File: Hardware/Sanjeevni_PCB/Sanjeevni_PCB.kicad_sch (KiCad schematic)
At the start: 45 parts, among them J1 Conn_01x02, J2 Conn_01x04, J3 Conn_01x04, SW1 SW_Push, SW2 SW_Push, U1 AMS1117-3.3, U2 MT3608, U3 ADXL343, U4 ESP32-WROOM-32, U5 DHT11, U6 MQ-6

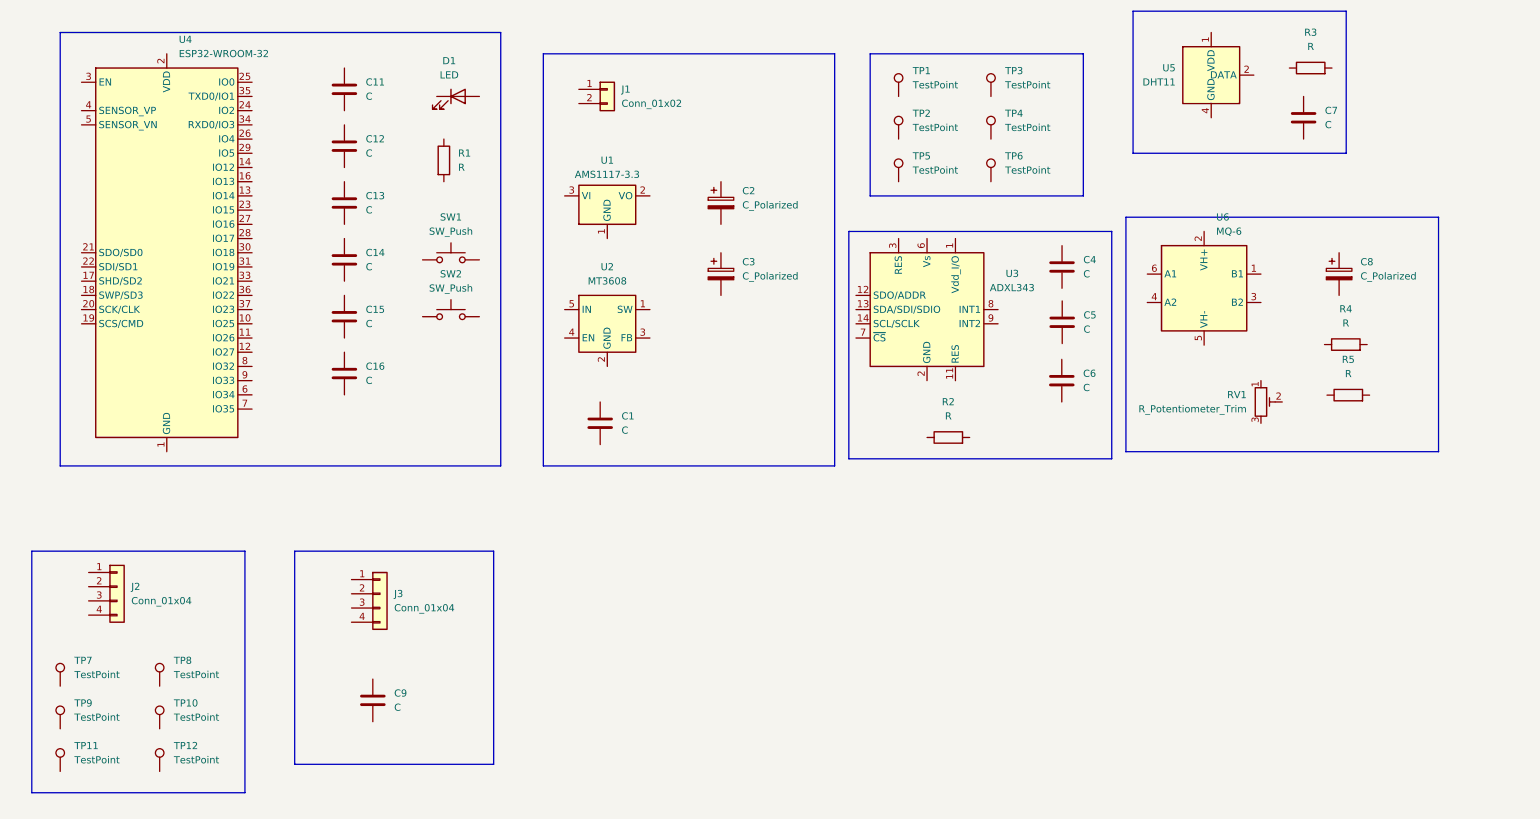
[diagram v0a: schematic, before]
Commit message: final PCB design KiCad
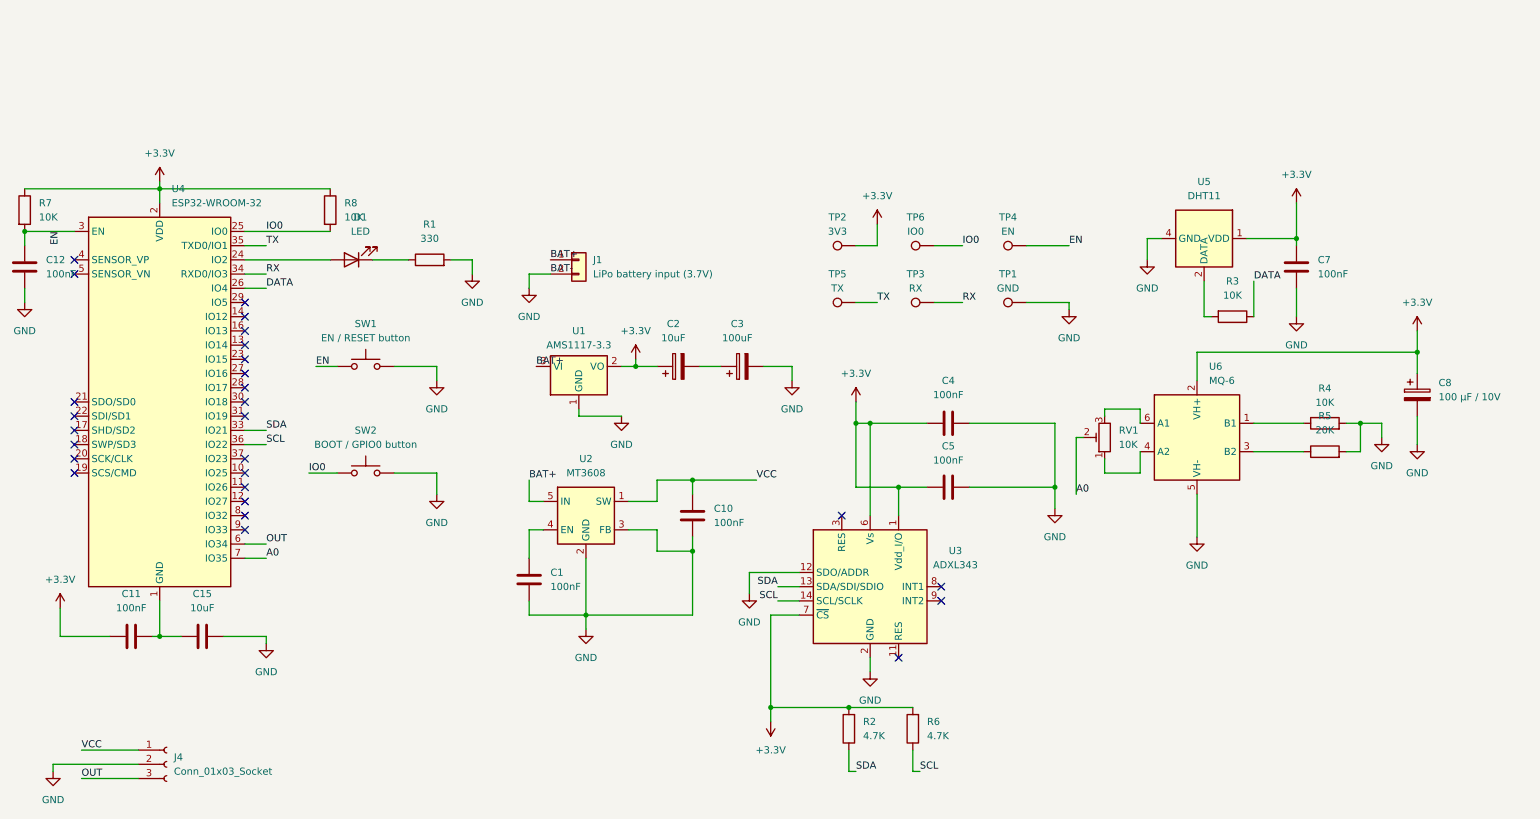
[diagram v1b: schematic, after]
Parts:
- removed C13, C14, C16, C6, C9: C, Capacitor_SMD:C_0402_1005Metric, symbol Device:C
- removed J2, J3: Conn_01x04, Connector:FanPinHeader_1x04_P2.54mm_Vertical, symbol Connector_Generic:Conn_01x04
- removed TP10, TP11, TP12, TP7, TP8, TP9: TestPoint, TestPoint:TestPoint_Pad_1.5x1.5mm, symbol Connector:TestPoint
- added C10: 100nF, Capacitor_SMD:C_0402_1005Metric, symbol Device:C
- added J4: Conn_01x03_Socket, Connector_PinSocket_2.00mm:PinSocket_1x03_P2.00mm_Horizontal, symbol Connector:Conn_01x03_Socket
- added R6: 4.7K, Resistor_SMD:R_0402_1005Metric, symbol Device:R
- added R7, R8: 10K, Resistor_SMD:R_0402_1005Metric, symbol Device:R
- C1, C11, C12, C4, C5, C7: value C -> 100nF
- C15: value C -> 10uF
- C2: value C_Polarized -> 10uF
- C3: value C_Polarized -> 100uF
- C8: value C_Polarized -> 100 µF / 10V
- J1: value Conn_01x02 -> LiPo battery input (3.7V)
- R1: value R -> 330
- R2: value R -> 4.7K
- R3, R4: value R -> 10K
- R5: value R -> 20K
- RV1: value R_Potentiometer_Trim -> 10K
- SW1: value SW_Push -> EN / RESET button
- SW2: value SW_Push -> BOOT / GPIO0 button
- TP1: value TestPoint -> GND
- TP2: value TestPoint -> 3V3
- TP3: value TestPoint -> RX
- TP4: value TestPoint -> EN
- TP5: value TestPoint -> TX
- TP6: value TestPoint -> IO0
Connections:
- net +3.3V: now reaches U3.1 (Vdd_I/O)
- net +3.3V: now also C11.1, C2.1, C4.1, C5.1, C7.1, C8.1, R2.2, TP2.1, U1.2 (VO), U3.6 (Vs), U3.7 (~{CS}), U4.2 (VDD), U5.1 (VDD), U6.2 (VH+), R6.2, R7.1, R8.1
- net GND: now reaches U3.12 (SDO/ADDR)
- net GND: now also C1.2, C12.2, C15.2, C3.2, C4.2, C5.2, C7.2, C8.2, J1.2 (Pin_2), R1.2, R4.2, R5.2, SW1.2, SW2.2, TP1.1, U1.1 (GND), U2.2 (GND), U2.3 (FB), U3.2 (GND), U3.4 (GND), U3.5 (GND), U5.4 (GND), U6.5 (VH-), C10.2, J4.2 (Pin_2)
- net SDA: now reaches U3.13 (SDA/SDI/SDIO)
- net SDA: now also R2.1, U4.33 (IO21)
- net SCL: now reaches U3.14 (SCL/SCLK)
- net SCL: now also U4.36 (IO22), R6.1
- net at R1.1: now also D1.1 (K)
- net RX: now reaches TP3.1
- net RX: now also U4.34 (RXD0/IO3)
- net BAT+: now reaches J1.1 (Pin_1)
- net BAT+: now also U1.3 (VI), U2.5 (IN)
- net EN: now reaches TP4.1
- net EN: now also C12.1, SW1.1, U4.3 (EN), R7.2
- net at R4.1: now also U6.1 (B1)
- net at U4.1 (GND), U4.15 (GND), U4.38 (GND)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: now also C11.2, C15.1
- net at U4.24 (IO2): now also D1.2 (A)
- net IO0: now reaches U4.25 (IO0)
- net IO0: now also SW2.1, TP6.1, R8.2
- net DATA: now reaches U4.26 (IO4)
- net DATA: now also R3.1
- net TX: now reaches U4.35 (TXD0/IO1)
- net TX: now also TP5.1
- net OUT: now reaches U4.6 (IO34)
- net OUT: now also J4.3 (Pin_3)
- net A0: now reaches U4.7 (IO35)
- net A0: now also RV1.2
- net at U6.3 (B2): now also R5.1
- net at U6.4 (A2): now also RV1.1
- net at U6.6 (A1): now also RV1.3
- net at C1.1: now also U2.4 (EN)
- net at C2.2: now also C3.1
- net at U5.2 (DATA): now also R3.2
- net VCC: now reaches U2.1 (SW)
- net VCC: now also C10.1, J4.1 (Pin_1)
- no-connect marks 0 -> 27
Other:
- moved on the sheet: C1, C11, C12, C15, C2, C3, C4, C5, C7, C8, D1, J1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
